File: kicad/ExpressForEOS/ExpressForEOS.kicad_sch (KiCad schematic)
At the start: 17 parts, among them J1 Conn_02x17_Counter_Clockwise, U1 74HC4051, U10 74LS08, U11 74LS156, U12 74LS156, U13 74LS373, U14 ICM7218BIPI, U15 MAX150BCPP, U16 LM358, U2 74HC4051, U3 74HC4051, U4 74HC4051, U5 CD4066BE, U6 74LS138, U7 74LS374, U8 74LS374, U9 74LS245

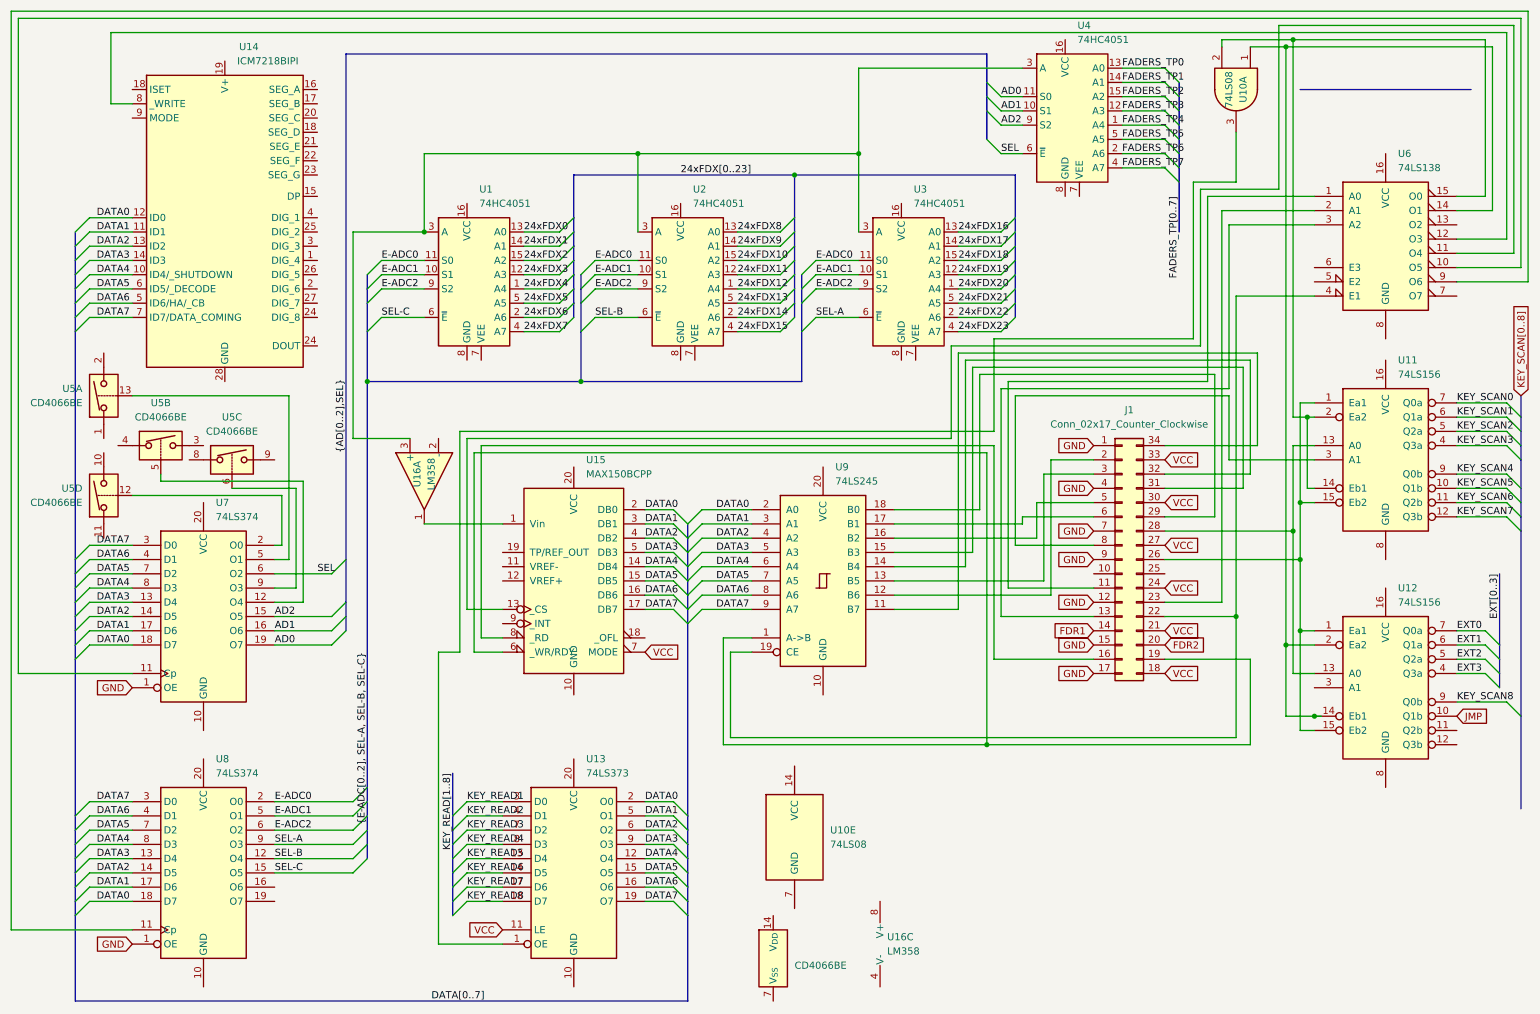
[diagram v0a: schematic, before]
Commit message: More tidy-up work
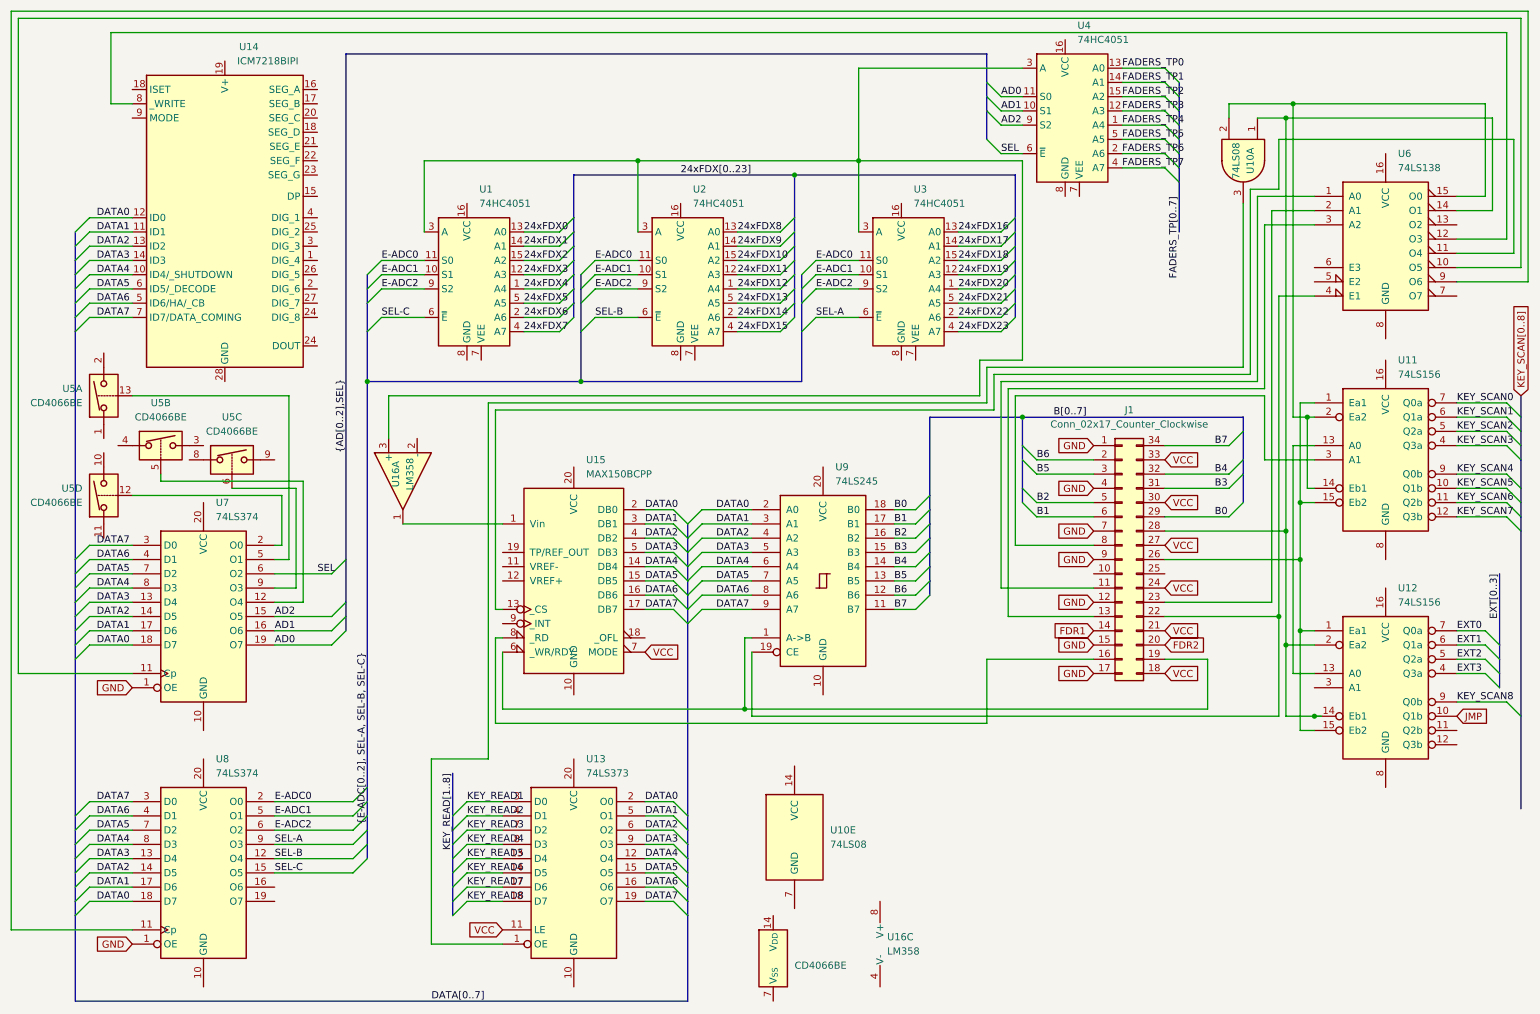
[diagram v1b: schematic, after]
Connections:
- net at U11.13 (A0), U12.13 (A0): no longer J1.28 (Pin_28)
- net at U10.1, U12.14 (Eb1), U12.2 (Ea2)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: now also J1.28 (Pin_28)
- net B7: now reaches J1.34 (Pin_34), U9.11 (B7)
- net B6: now reaches J1.2 (Pin_2), U9.12 (B6)
- net B5: now reaches J1.3 (Pin_3), U9.13 (B5)
- net B4: now reaches J1.32 (Pin_32), U9.14 (B4)
- net B3: now reaches J1.31 (Pin_31), U9.15 (B3)
- net B2: now reaches J1.5 (Pin_5), U9.16 (B2)
- net B1: now reaches J1.6 (Pin_6), U9.17 (B1)
- net B0: now reaches J1.29 (Pin_29), U9.18 (B0)
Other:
- moved on the sheet: U10A, U16A
